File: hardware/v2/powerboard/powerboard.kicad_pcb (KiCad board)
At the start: 2 copper layers, 52.7 x 66 mm, 35 parts, among them J1 LEG1_PWR, J10 UBEC3, J11 SBEC, J12 LOGIC_5V_OUT, J13 MONITOR, J2 LEG2_PWR, J3 LEG3_PWR, J4 LEG4_PWR, J5 LEG5_PWR, J6 LEG6_PWR, J7 BATTERY, J8 UBEC1, J9 UBEC2, Q1 FQP47P06, Q2 FQP47P06, Q3 MMBT3904

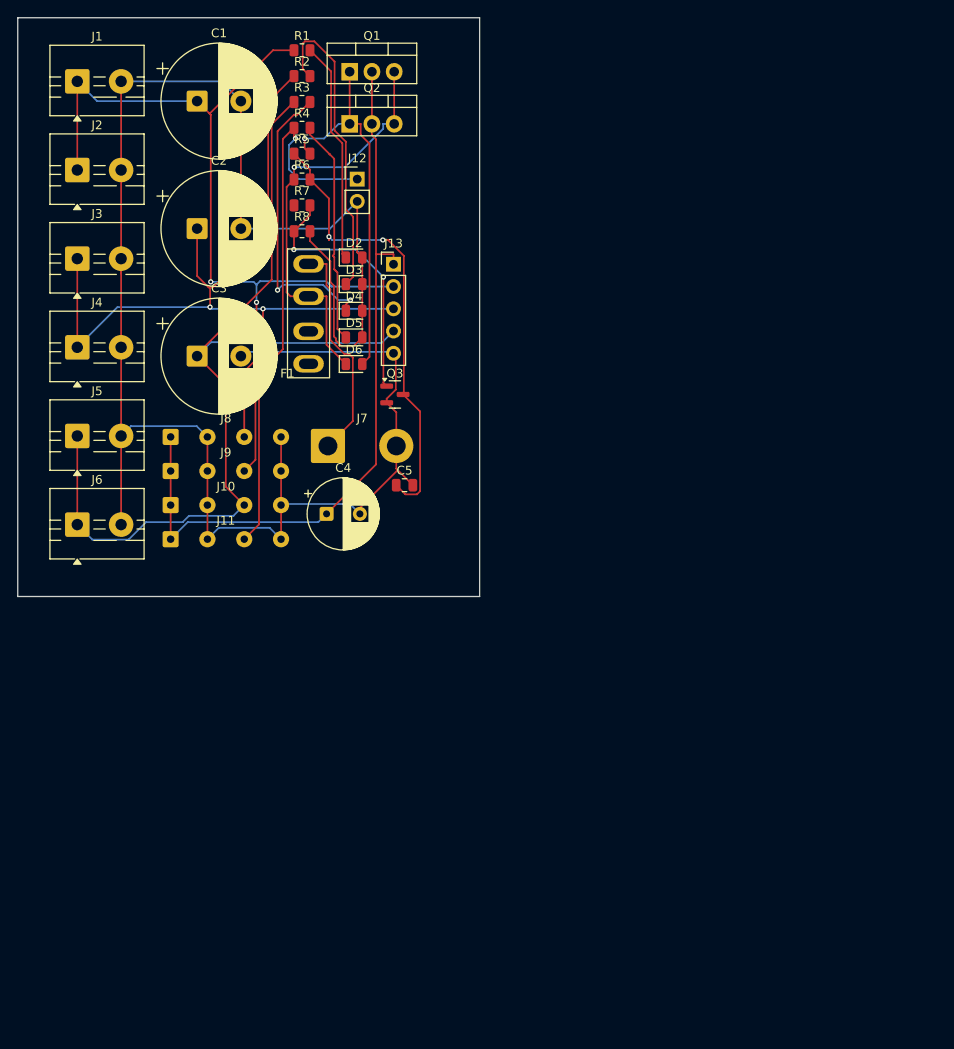
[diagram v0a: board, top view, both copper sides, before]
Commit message: powerboard layout
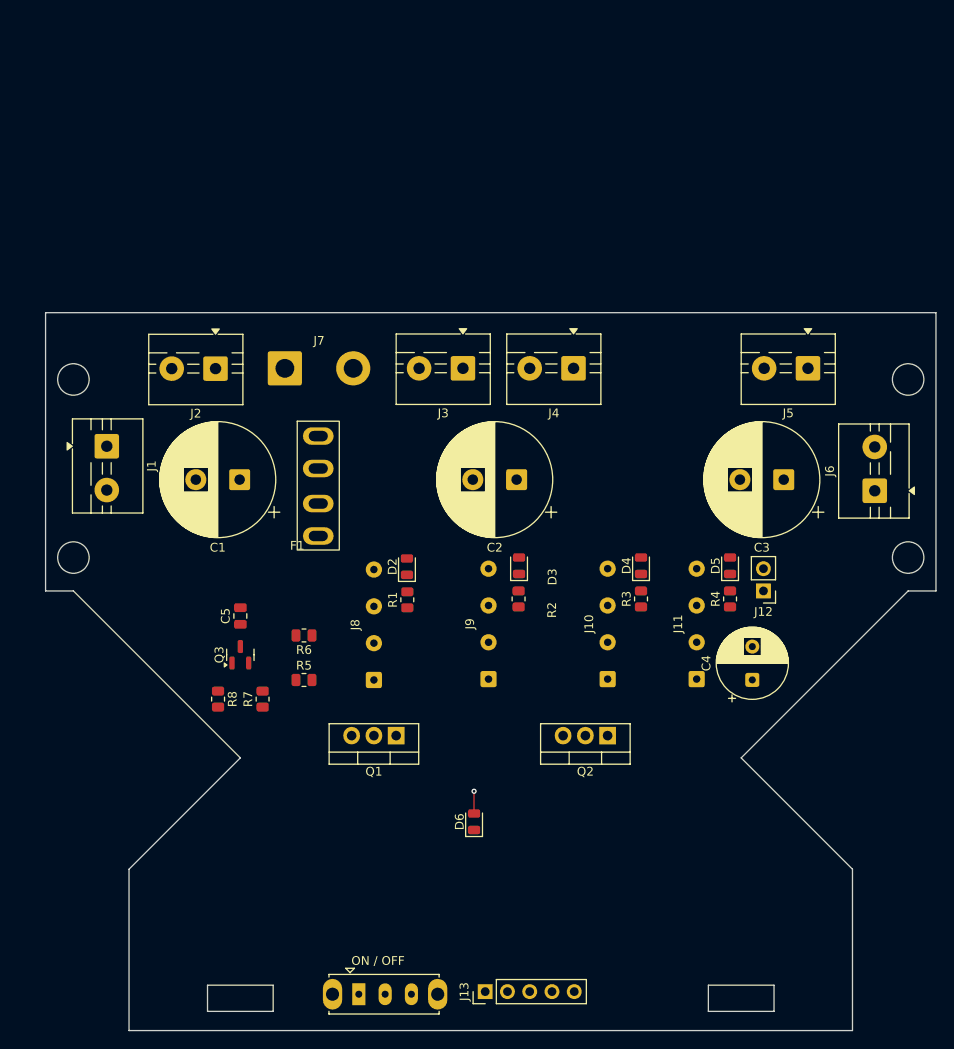
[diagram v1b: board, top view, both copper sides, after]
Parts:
- added ON / OFF: MASTER_SW, Custom:SW_Slide_SPDT_Straight, F.Cu at (82.4, 128.6)
- moved J6 91.1 mm to (142.2, 71.1), turned to 90 degrees
- moved J5 83.7 mm to (134.6, 57.1), turned to 180 degrees
- moved J13 83.7 mm to (97.8, 128.3), turned to 90 degrees
- moved Q1 75.9 mm to (87.6, 99.1), turned to 180 degrees
- moved Q2 75.8 mm to (111.8, 99.1), turned to 180 degrees
- moved R4 72.6 mm to (125.7, 83.5), turned to 90 degrees
- moved R3 68.6 mm to (115.6, 83.5), turned to 90 degrees
- moved C3 68.4 mm to (131.9, 69.8), turned to 180 degrees
- moved J12 66.0 mm to (129.5, 82.5), turned to 180 degrees
- moved R2 64.6 mm to (101.6, 83.5), turned to 90 degrees
- moved R1 63.8 mm to (88.9, 83.6), turned to 90 degrees
- moved J11 62.1 mm to (121.9, 92.6), turned to 90 degrees
- moved R5 60.1 mm to (77.1, 92.7)
- moved J4 56.7 mm to (107.9, 57.1), turned to 180 degrees
- moved R7 56.5 mm to (72.4, 94.9), turned to 90 degrees
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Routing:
- net GND: track 223.6 -> 0.00 mm
- net VSERVO3: track 108.0 -> 0.00 mm
- net VSERVO2: track 105.5 -> 0.00 mm, vias 2 -> 0
- net VSERVO1: track 98.0 -> 0.00 mm, vias 2 -> 0
- net +VMAIN: track 86.8 -> 0.00 mm
- net +5V: track 62.7 -> 0.00 mm, vias 1 -> 0
- net PMOS_GATE_DRV: track 53.0 -> 0.00 mm, vias 2 -> 0
- net BATT_FUSED: track 47.7 -> 0.00 mm, vias 1 -> 0
- net PMOS_GATE: track 43.2 -> 2.54 mm
- net LED_U2: track 35.4 -> 0.00 mm
- net LED_U3: track 33.9 -> 0.00 mm, vias 2 -> 0
- net NPN_BASE: track 29.9 -> 0.00 mm, vias 2 -> 0
- net LED_SBEC: track 26.3 -> 0.00 mm
- net BATT_RAW: track 25.6 -> 0.00 mm
- net LED_U1: track 25.3 -> 0.00 mm
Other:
- board size 52.7 x 66 mm -> 101.6 x 81.9 mm
